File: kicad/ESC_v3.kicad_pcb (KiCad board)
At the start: 6 copper layers, 50 x 35 mm, 98 parts, among them J1 Conn_01x07, J10 Conn_01x03, J2 Conn_01x05_Pin, J3 USB_C_Receptacle_USB2.0, J4 Conn_01x04, J6 Conn_01x06_Pin, J7 Conn_01x02_Pin, J8 Conn_01x04_Pin, J9 Conn_01x02, Q1 RH6L040BGTB1, Q3 RH6L040BGTB1, Q4 RH6L040BGTB1, Q5 RH6L040BGTB1, Q6 RH6L040BGTB1, Q7 RH6L040BGTB1, SW2 SW_Nidec_CAS-120A1, U1 STSPIN32G4, U10 BD4104, U14 MCP9700x-ETT, U2 AMS1117-5.0, X1 IQXO-70

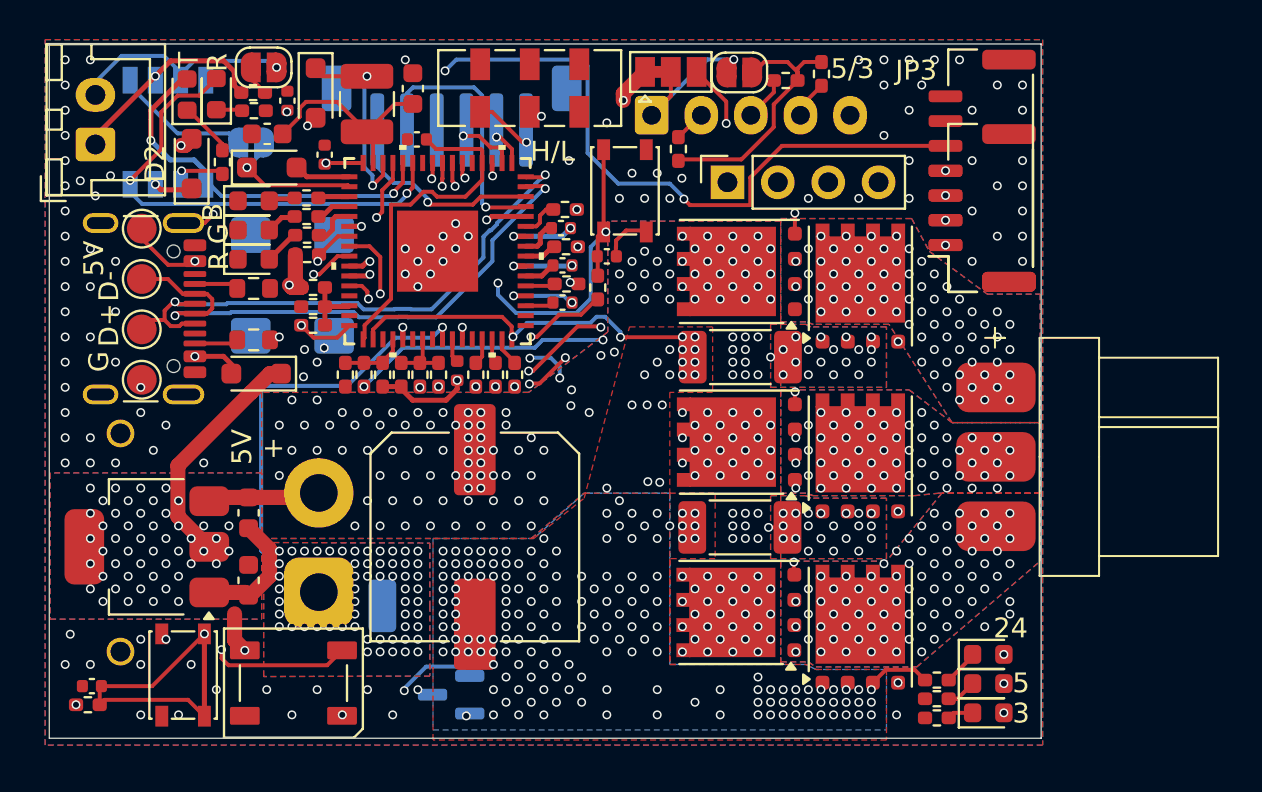
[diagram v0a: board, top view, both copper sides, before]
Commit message: add v2_mini_mini
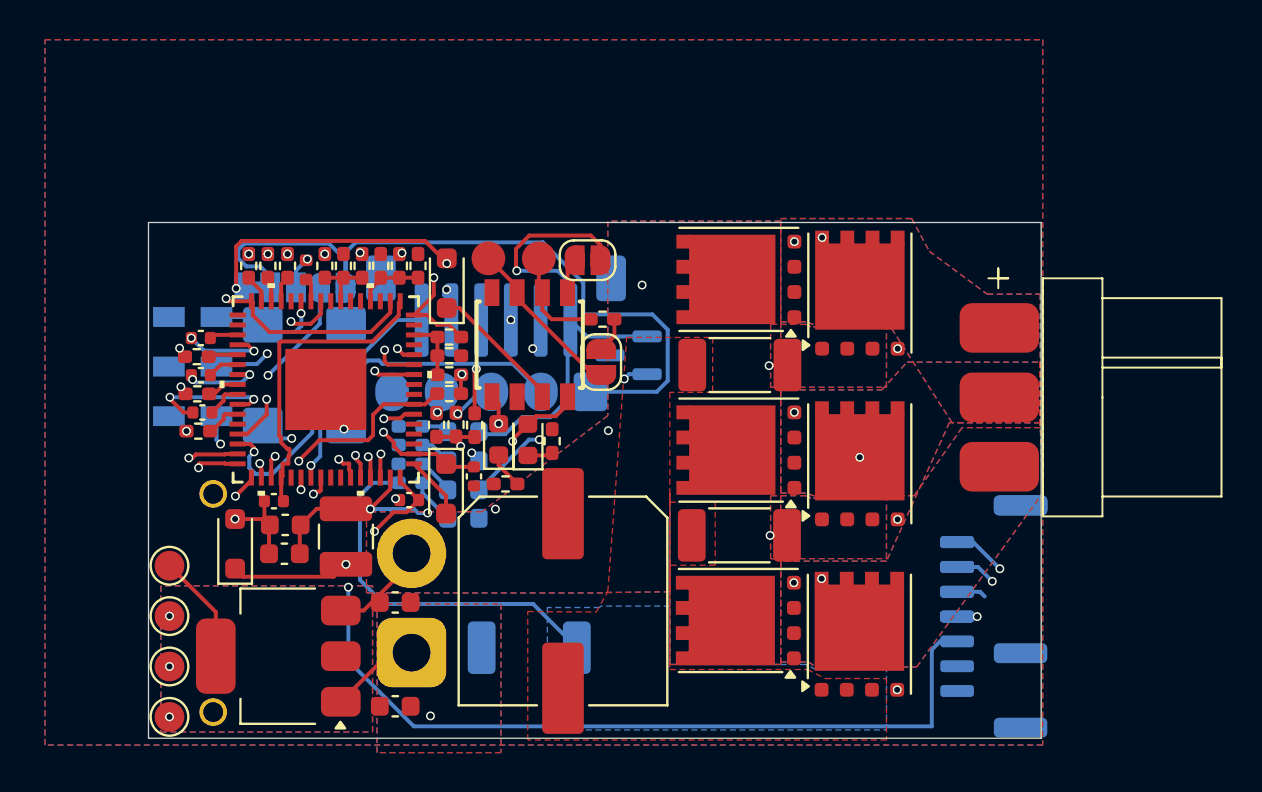
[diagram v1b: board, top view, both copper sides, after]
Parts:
- removed C23, C39: 0.1u, Capacitor_SMD:C_0402_1005Metric
- removed D14: WS2812B, LED_SMD:LED_WS2812B_PLCC4_5.0x5.0mm_P3.2mm
- removed D3: 1N5819WS, Diode_SMD:D_SOD-323_HandSoldering
- removed D4: LED_B, LED_SMD:LED_0603_1608Metric
- removed D5: LED_G, LED_SMD:LED_0603_1608Metric
- removed D6: LED_R, LED_SMD:LED_0603_1608Metric
- removed J3: USB_C_Receptacle_USB2.0, Connector_USB:USB_C_Receptacle_GCT_USB4105-xx-A_16P_TopMnt_Horizontal
- removed J8: Conn_01x04_Pin, Connector_PinSocket_2.54mm:PinSocket_1x04_P2.54mm_Vertical
- removed NRST1, button1: SW_Push, Button_Switch_SMD:SW_SPST_PTS810
- removed R21, R22, R25: 2.2k, Resistor_SMD:R_0402_1005Metric_Pad0.72x0.64mm_HandSolder
- removed R23, R24: 5.1k, Resistor_SMD:R_0603_1608Metric
- removed R5, R6: 10k, Resistor_SMD:R_0402_1005Metric_Pad0.72x0.64mm_HandSolder
- added D13: LED_R, LED_SMD:LED_0603_1608Metric, B.Cu at (70.9, 72.5)
- added R35: 10k, Resistor_SMD:R_0402_1005Metric_Pad0.72x0.64mm_HandSolder, B.Cu at (68.2, 71.2)
- D10, D11, D12, J1, J4, JP1, JP3, R27, R28, R30, SW2: moved to B.Cu
- J7: footprint Connector_JST:JST_XH_B2B-XH-A_1x02_P2.50mm_Vertical -> jisaku:名称未設定_1
- JP4, U10: moved to F.Cu
- moved G*** 59.9 mm to (17.8, 54.8), turned to 0 degrees
- moved G*** 58.8 mm to (17.7, 58.2), turned to 0 degrees
- moved G*** 51.5 mm to (21.3, 63.6), turned to 0 degrees
- moved G*** 46.4 mm to (24.1, 57.6), turned to 0 degrees
- moved R30 30.3 mm to (68.2, 69.3)
- moved D12 30.0 mm to (70.9, 69.5)
- moved R28 29.5 mm to (68.2, 70.2)
- moved D11 28.7 mm to (70.9, 71.0)
- moved R27 28.3 mm to (68.2, 72.1)
- moved D10 27.3 mm to (70.9, 73.9)
- moved R33 26.3 mm to (69.5, 69.2), turned to 90 degrees
- moved C1 24.3 mm to (61.9, 75.7), turned to 180 degrees
- moved R32 24.0 mm to (70.5, 69.2), turned to 90 degrees
- moved D8 23.5 mm to (74.1, 70.0)
- moved D9 23.4 mm to (72.7, 69.9)
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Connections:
- net Net-(U1-VCC) renamed VCC
- C1 pad 2: OPAMP3_VINM -> GND
- C11 pad 2: OPAMP3_VINM -> GND
- C6 pad 2: OPAMP3_VINM -> GND
- C7 pad 2: OPAMP3_VINM -> GND
- C8 pad 2: OPAMP3_VINM -> GND
- D1 pad 2: OPAMP3_VINM -> GND
- J1 pad 3: OPAMP3_VINM -> GND
- J2 pad 5: OPAMP3_VINM -> GND
- J4 pad 3: OPAMP3_VINM -> GND
- J6 pad 4: OPAMP3_VINM -> GND
- Q3 pad 1: /power_stage/GND -> OPAMP1_VINM
- Q7 pad 1: OPAMP1_VINM -> /power_stage2/GND
- R12 pad 1: /power_stage/GND -> /power_stage2/GND
- R13 pad 2: +3.3V -> unconnected-(R13-Pad2)
- R14 pad 1: OPAMP3_VINM -> GND
- R17 pad 1: OPAMP3_VINM -> GND
- R20 pad 1: OPAMP3_VINM -> GND
- R26 pad 1: OPAMP3_VINM -> GND
- R28 pad 1: OPAMP3_VINM -> GND
- R29 pad 1: OPAMP3_VINM -> GND
- R30 pad 1: OPAMP3_VINM -> GND
- R8 pad 1: /power_stage/GND -> /power_stage2/GND
- SW2 pad 1: OPAMP3_VINM -> GND
- TP1 pad 1: Net-(D3-A) -> +5V
- TP4 pad 1: OPAMP3_VINM -> GND
- U1 pad 65: OPAMP3_VINM -> GND
- U10 pad 2: OPAMP3_VINM -> GND
- U10 pad 8: OPAMP3_VINM -> GND
- U14 pad 3: OPAMP3_VINM -> GND
- X1 pad 2: OPAMP3_VINM -> GND
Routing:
- net +5V: track 108.9 -> 49.3 mm, vias 53 -> 4
- net button: track 41.2 -> 0.00 mm, vias 2 -> 0
- net TIM4_CH2: track 38.0 -> 0.00 mm, vias 2 -> 0
- net +15V: track 42.8 -> 11.9 mm, vias 179 -> 3
- net Net-(J2-Pin_1): track 7.89 -> 37.9 mm, vias 1 -> 0
- net OPAMP3_VINM: track 63.6 -> 33.9 mm, vias 170 -> 1
- net NRST: track 29.2 -> 0.00 mm, vias 3 -> 0
- net /power_stage/OUT: track 16.8 -> 45.2 mm, vias 72 -> 3
- net Net-(Q3-G): track 23.4 -> 51.5 mm, vias 4 -> 2
- net I2C_SCL: track 26.0 -> 0.00 mm, vias 1 -> 0
- net +3.3V: track 72.8 -> 98.2 mm, vias 13 -> 7
- net Net-(Q1-G): track 12.1 -> 36.8 mm
- net /power_stage/GND: track 24.0 -> 0.00 mm, vias 20 -> 0
- net I2C_SDA: track 23.9 -> 0.00 mm, vias 1 -> 0
- net ADC1_IN9: track 36.9 -> 14.3 mm
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- added copper zone on B.Cu, net /power_stage2/GND
- added copper zone on F.Cu, net /power_stage2/GND
- added copper zone on In1.Cu, net /power_stage2/GND
- added copper zone on In2.Cu, net /power_stage2/GND
- added copper zone on In3.Cu, net /power_stage2/GND
- added copper zone on In4.Cu, net /power_stage2/GND
- added copper zone on B.Cu, net GND
- added copper zone on F.Cu, net GND
- added copper zone on In1.Cu, net GND
- added copper zone on In4.Cu, net GND
- removed copper zone on B.Cu, net /power_stage/GND
- removed copper zone on F.Cu, net /power_stage/GND
- removed copper zone on In1.Cu, net /power_stage/GND
- removed copper zone on In2.Cu, net /power_stage/GND
- removed copper zone on In3.Cu, net /power_stage/GND
- removed copper zone on In4.Cu, net /power_stage/GND
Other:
- board size 50 x 35 mm -> 45 x 26 mm
- board text removed: "+"
- board text removed: "24"
- board text removed: "3"
- board text removed: "5"
- board text removed: "5/3"
- board text removed: "5V"
- board text removed: "B"
- board text removed: "D+"
- board text removed: "D-"
- board text removed: "ESC_V2_mini"
- board text removed: "G"
- board text removed: "H/L"
- board text removed: "R"
- board text removed: "T"
- board text removed: "maked by k.r."
